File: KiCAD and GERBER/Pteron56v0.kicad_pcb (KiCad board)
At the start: 2 copper layers, 152.4 x 125.7 mm, 59 parts, among them J1 AudioJack4, J2 AudioJack4, SW1 SW_PUSH, SW10 SW_PUSH, SW11 SW_PUSH, SW12 SW_PUSH, SW13 SW_PUSH, SW14 SW_PUSH, SW15 SW_PUSH, SW16 SW_PUSH, SW17 SW_PUSH, SW18 SW_PUSH, SW19 SW_PUSH, SW2 SW_PUSH, SW20 SW_PUSH, SW21 SW_PUSH, SW22 SW_PUSH, SW23 SW_PUSH, SW24 SW_PUSH, SW25 SW_PUSH, SW26 SW_PUSH, SW27 SW_PUSH, SW28 SW_PUSH, SW3 SW_PUSH, SW4 SW_PUSH, SW5 SW_PUSH, SW6 SW_PUSH, SW7 SW_PUSH, SW8 SW_PUSH, SW9 SW_PUSH, U1 ProMicro

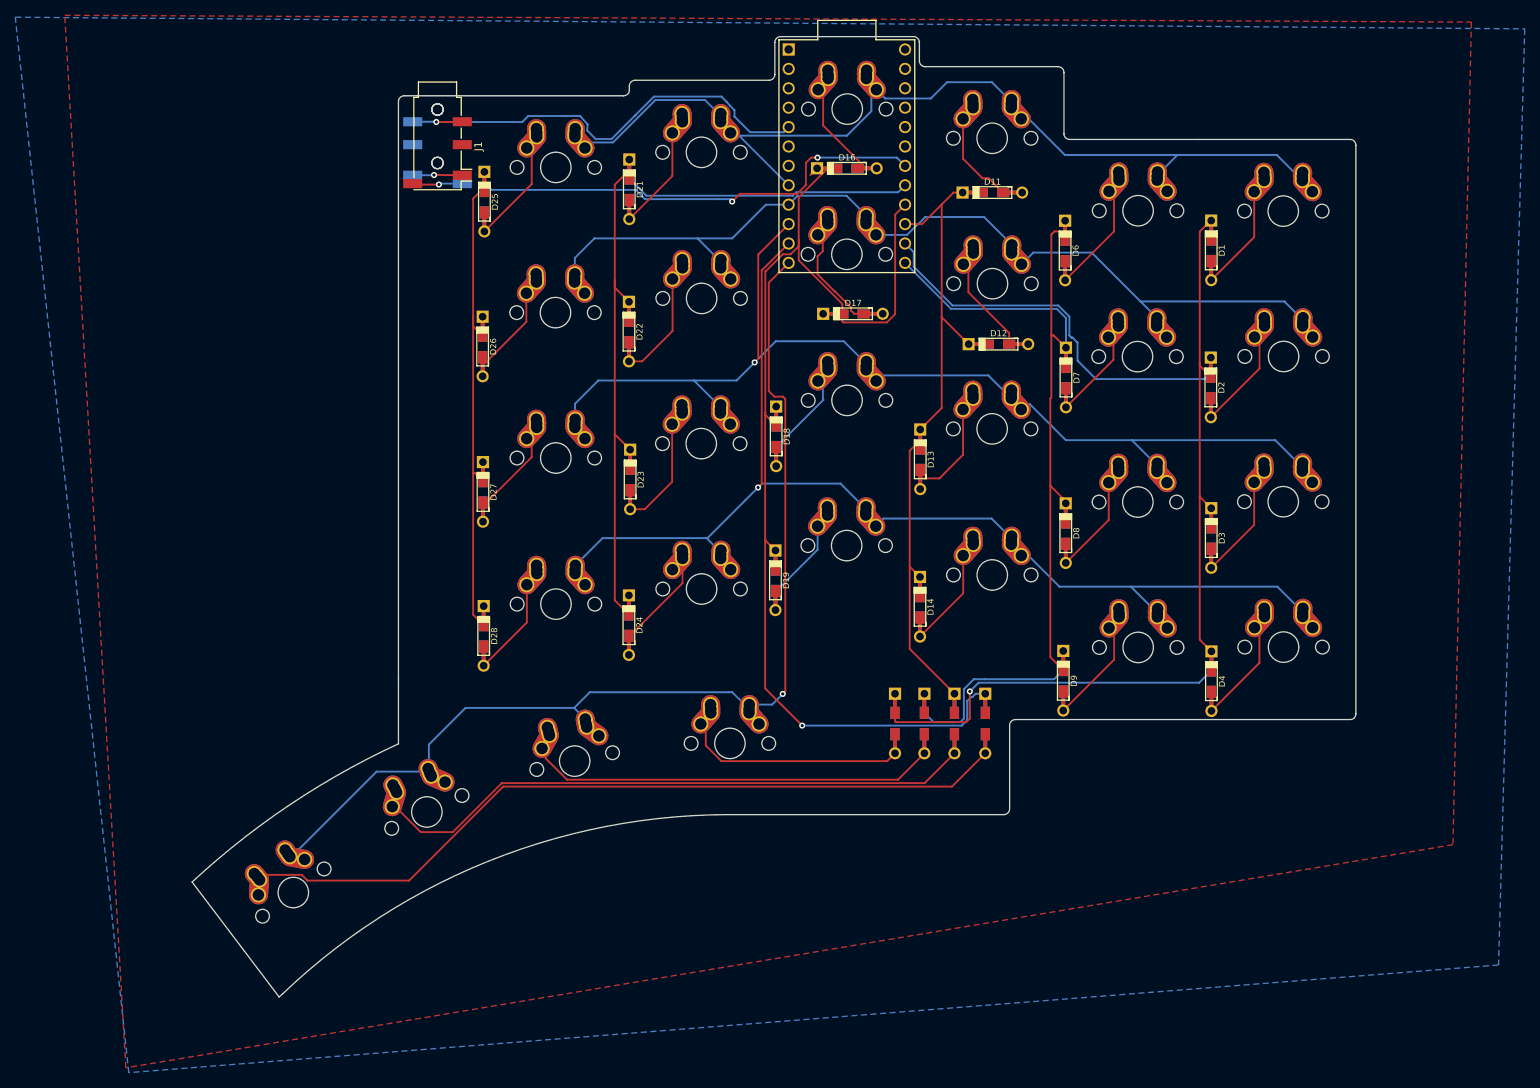
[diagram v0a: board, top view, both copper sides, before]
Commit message: split36 version
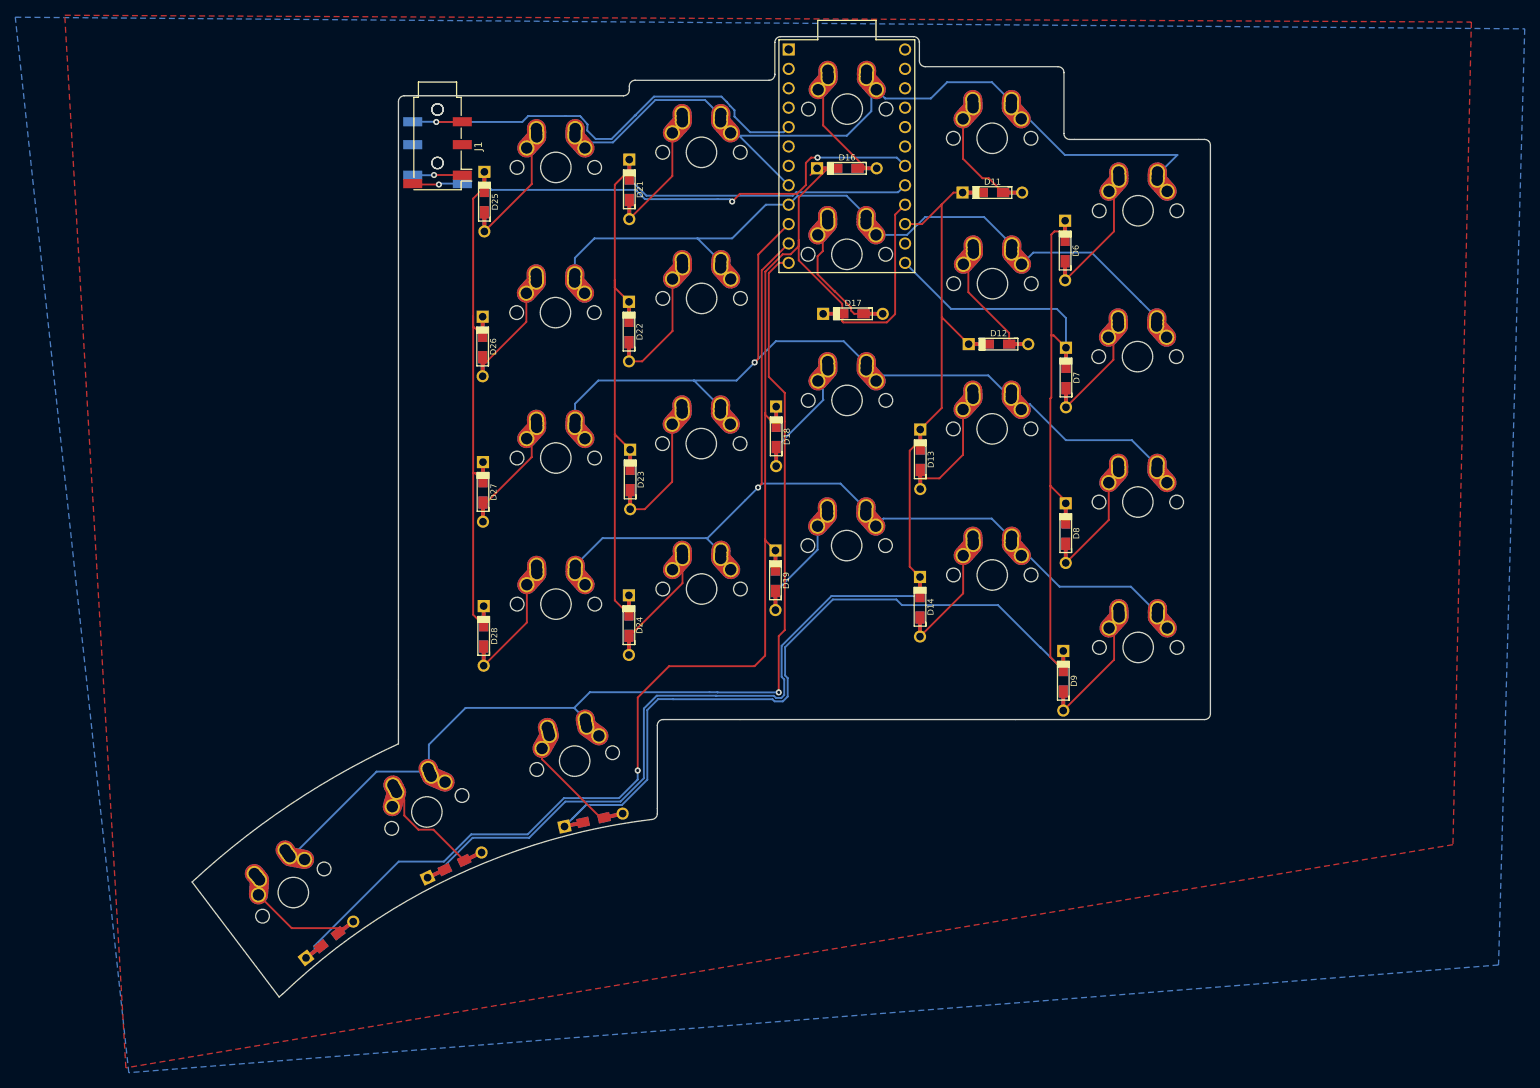
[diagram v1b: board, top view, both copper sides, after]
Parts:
- removed D1, D2, D3, D4, D5: 1N4148, Keebio-Parts:Diode-dual
- removed SW1, SW2, SW3, SW4, SW5: SW_PUSH, Keebio-Parts:Hybrid_PCB_100H_Dual_hole
- moved D20 90.4 mm to (91.8, 135.1), turned to 217.5 degrees
- moved D15 68.0 mm to (108.2, 125.3), turned to 205 degrees
- moved D10 45.1 mm to (126.4, 119.5), turned to 192.5 degrees
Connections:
- U1 pad 14: /Col0 -> (no net)
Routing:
- net /Col0: track 163.0 -> 0.00 mm, vias 1 -> 0
- net Net-(D20-Pad2): track 102.6 -> 13.1 mm
- net /Col1: track 117.2 -> 191.9 mm
- net /Col2: track 83.0 -> 152.0 mm
- net Net-(D15-Pad2): track 79.8 -> 13.8 mm
- net /Col3: track 148.1 -> 191.5 mm
- net Net-(D10-Pad2): track 54.3 -> 12.7 mm
- net Net-(D5-Pad2): track 29.6 -> 0.00 mm
- net /Row3: track 146.7 -> 121.2 mm
- net /Row2: track 135.1 -> 111.3 mm
- net /Row1: track 113.4 -> 91.2 mm
- net /Row0: track 122.7 -> 104.9 mm
- net Net-(D4-Pad2): track 14.2 -> 0.00 mm
- net Net-(D1-Pad2): track 13.9 -> 0.00 mm
- net Net-(D2-Pad2): track 13.9 -> 0.00 mm
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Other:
- board size 152.4 x 125.7 mm -> 133.3 x 125.7 mm
